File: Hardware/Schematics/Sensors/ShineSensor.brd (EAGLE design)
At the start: 15.2 x 20 mm, 6 parts

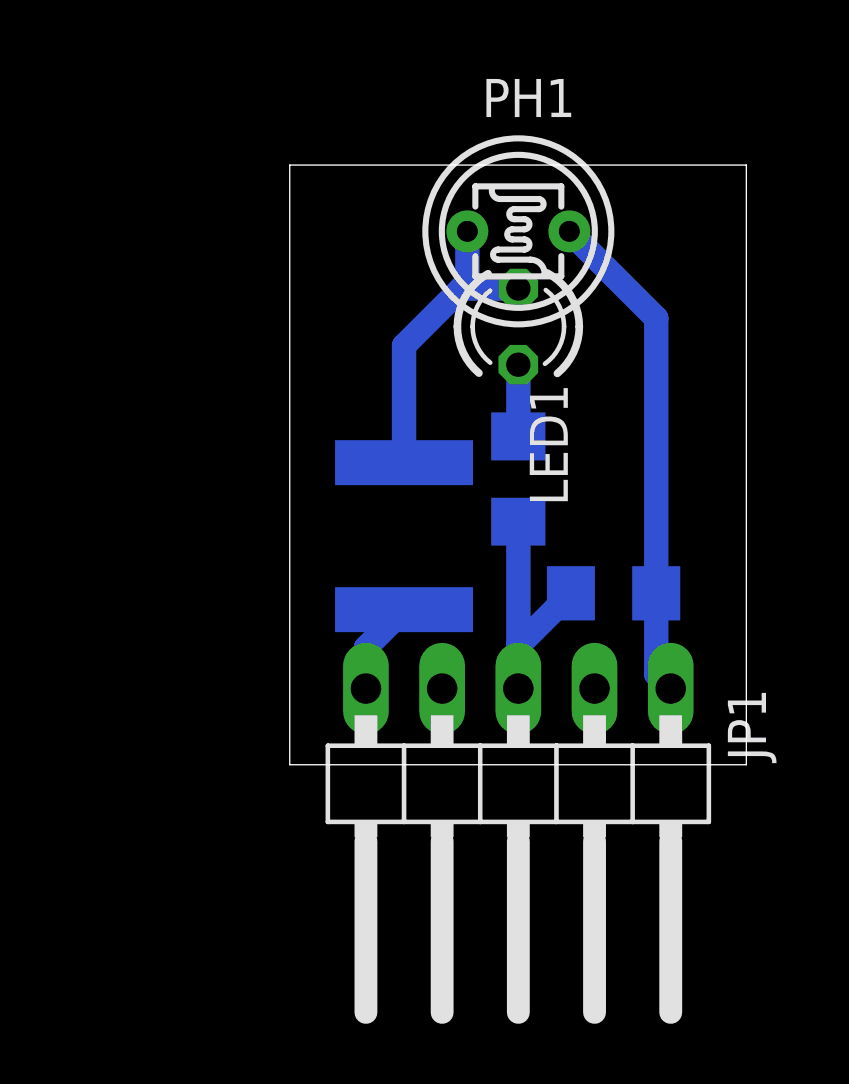
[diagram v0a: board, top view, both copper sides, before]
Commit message: sensors
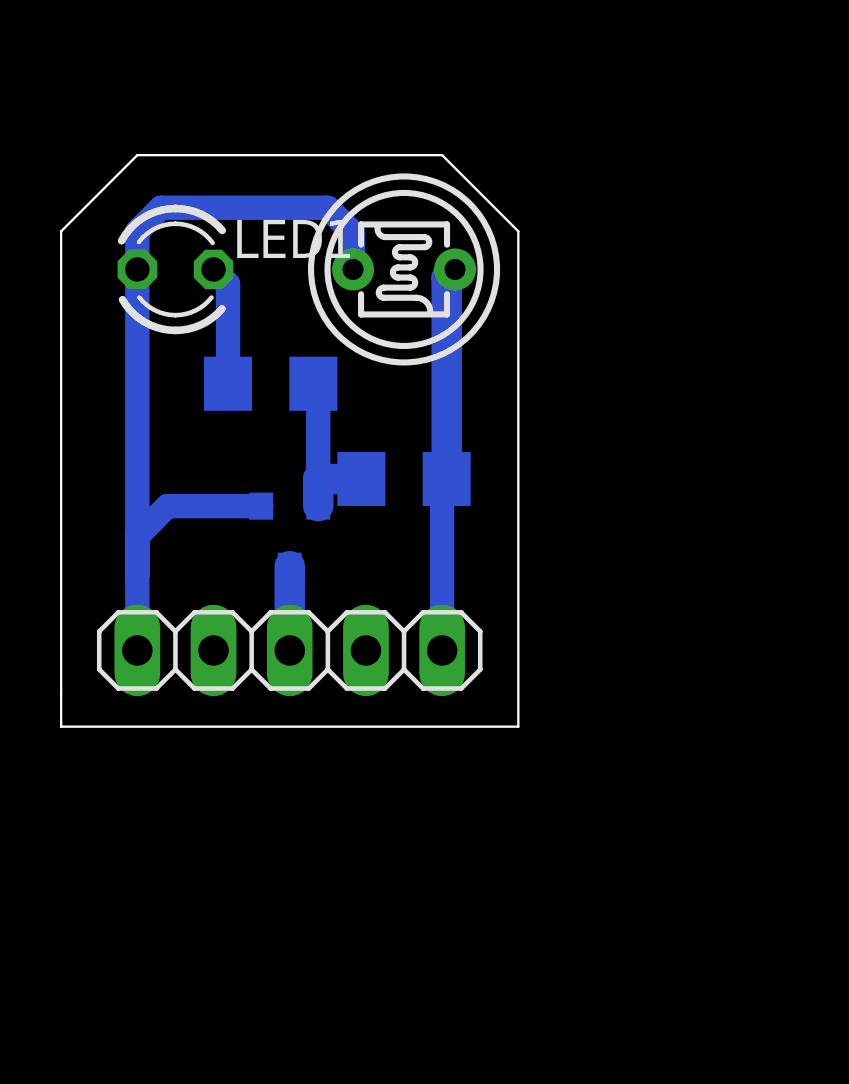
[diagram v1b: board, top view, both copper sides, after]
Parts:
- removed F1: 50ma, fuse:MF-SMDF050
- added Q1: BSS138, Cing Library:SOT23
- JP1: device pinhead:1X05/90 -> pinhead:1X05
- moved LED1 11.6 mm to (-3.81, 16.5), turned to 0 degrees
- moved JP1 9.16 mm to (0.00, 3.81)
- moved R2 8.84 mm to (-0.64, 12.7), turned to 0 degrees
- moved R1 7.96 mm to (3.81, 9.53)
- moved PH1 4.02 mm to (3.81, 16.5)
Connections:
- removed net N$15: F1.1, JP1.5
- new net N$3: JP1.3, Q1.3
- net N$1: now also JP1.5, Q1.1; no longer F1.2
- net N$14: now also Q1.2; no longer JP1.3
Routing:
- net N$1: track 10.5 -> 29.8 mm
- net N$14: track 9.46 -> 5.59 mm
- net N$13: track 16.6 -> 12.9 mm
- net N$15: track 3.16 -> 0.00 mm
- net N$3: track 0.00 -> 2.81 mm
- net N$2: track 2.39 -> 4.01 mm
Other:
- board size 15.2 x 20 mm -> 15.2 x 19.1 mm
